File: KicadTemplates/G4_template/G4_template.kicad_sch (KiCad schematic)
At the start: 13 parts, among them J1 Conn_01x04_Female, SW1 SW_SPDT, U1 NUCLEO-G491RE

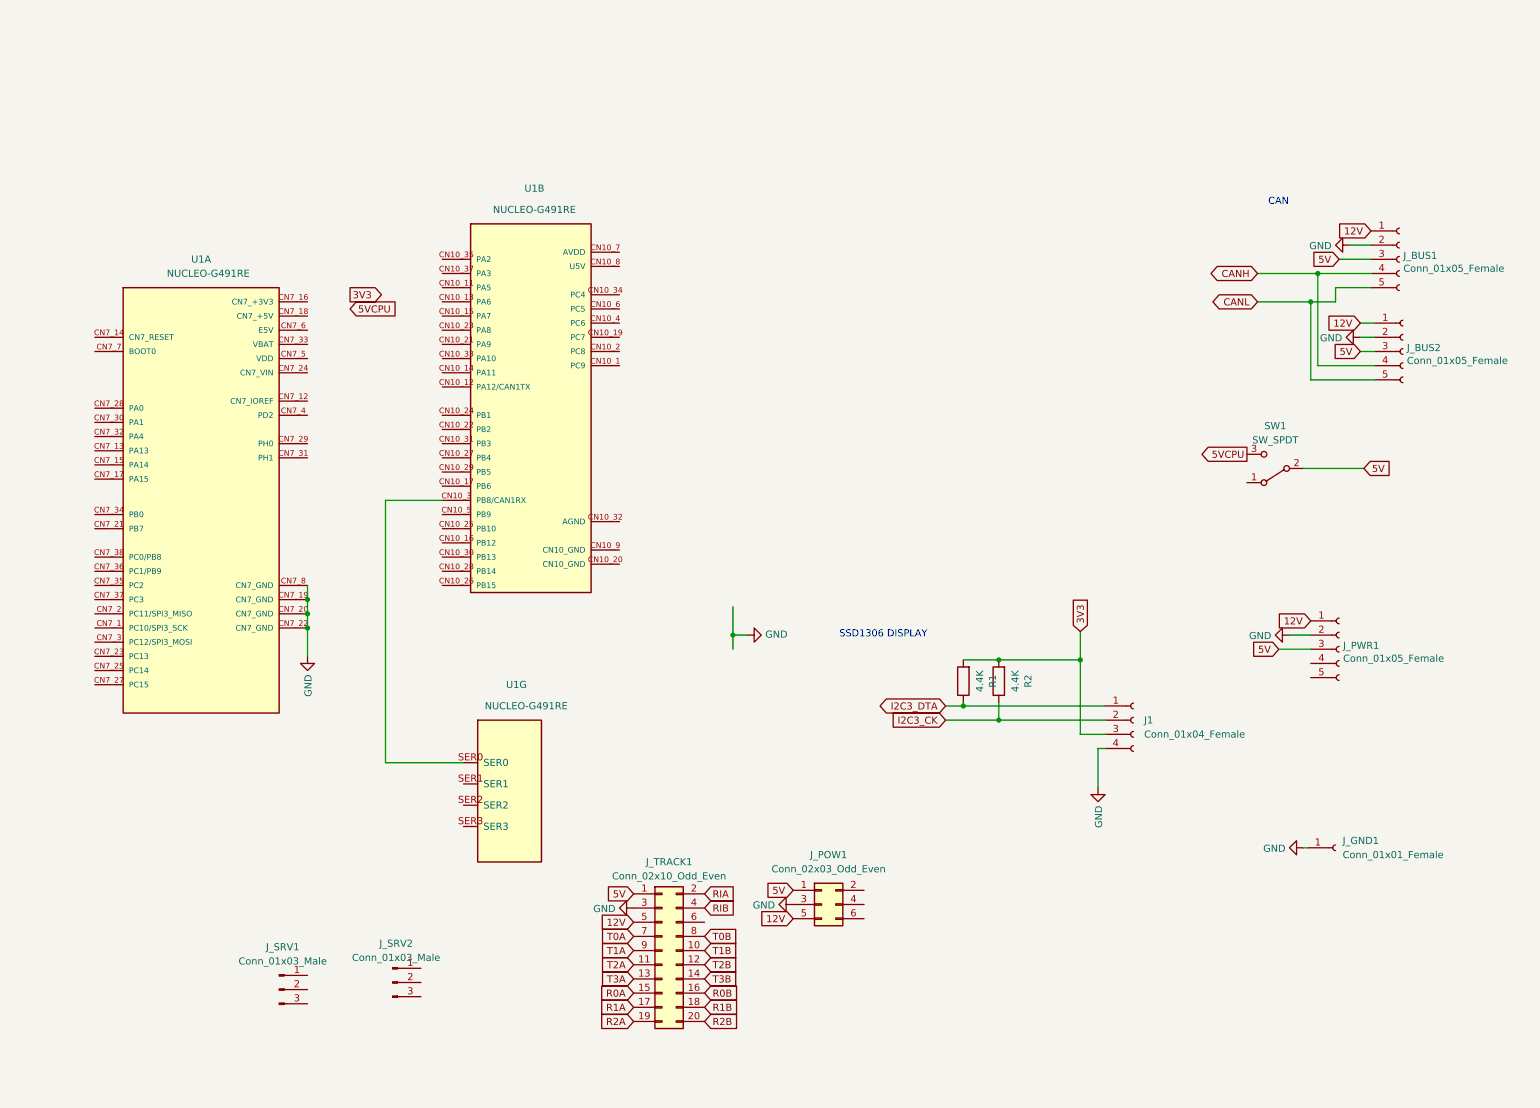
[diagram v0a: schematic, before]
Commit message: update spec
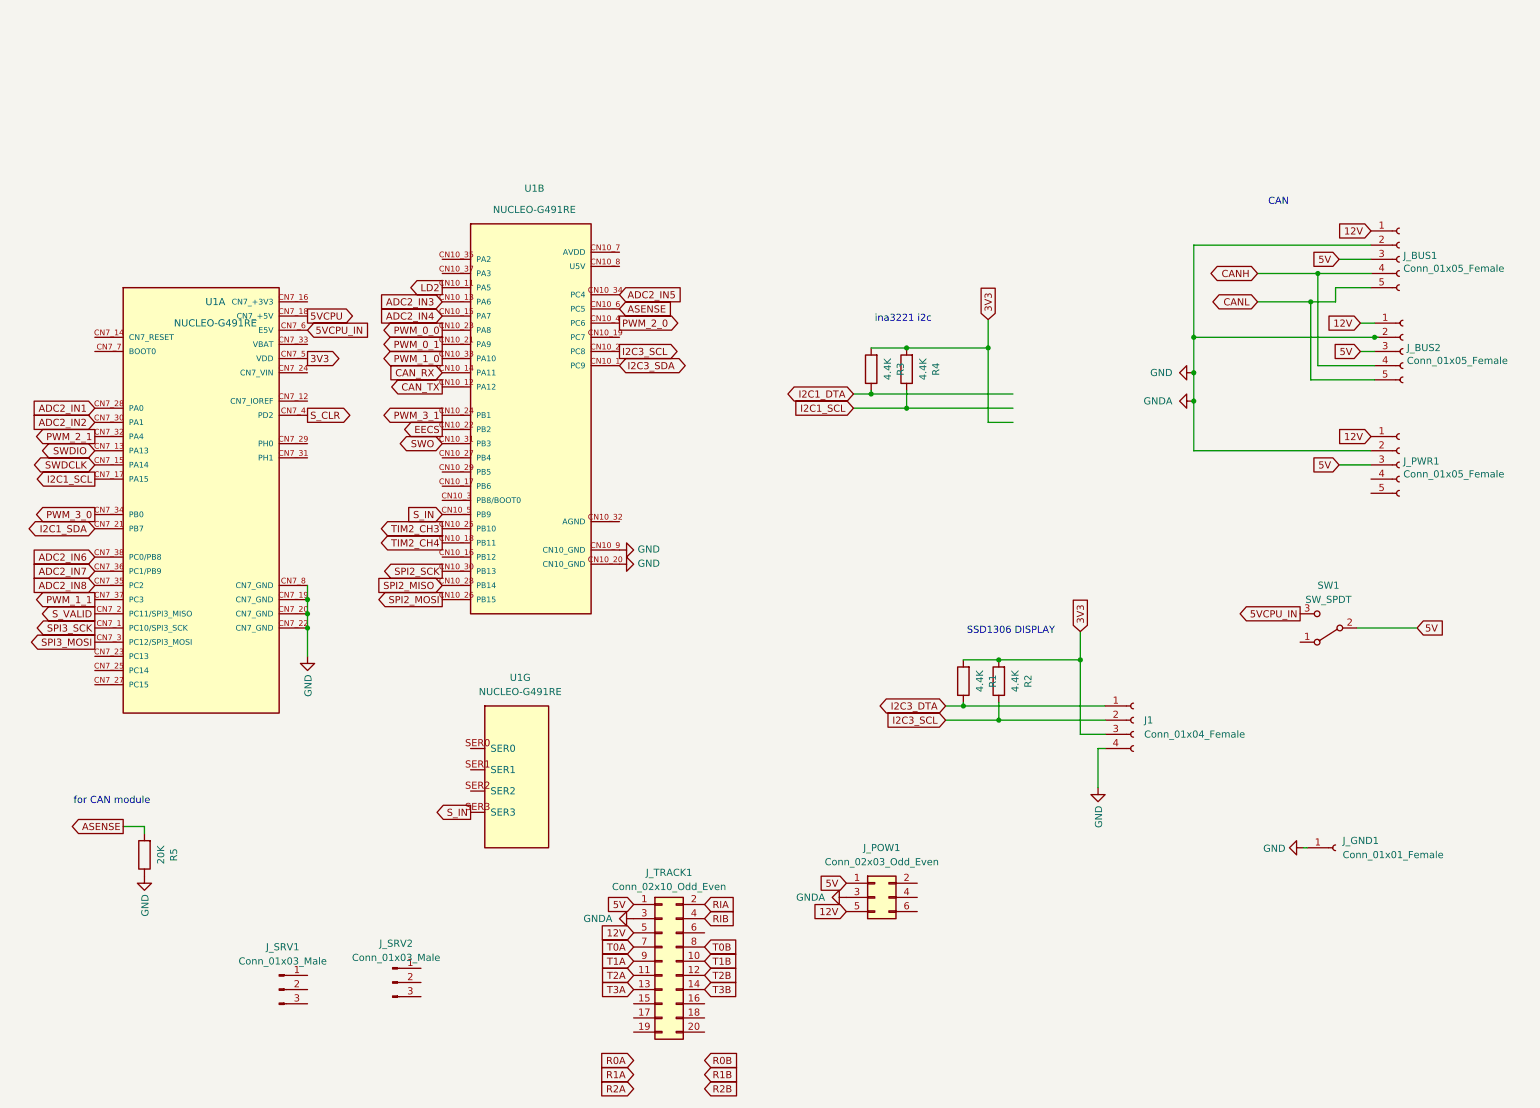
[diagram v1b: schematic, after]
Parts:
- added R3, R4: 4.4K, Resistor_THT:R_Axial_DIN0207_L6.3mm_D2.5mm_P7.62mm_Horizontal, symbol Device:R
- added R5: 20K, Resistor_THT:R_Axial_DIN0207_L6.3mm_D2.5mm_P7.62mm_Horizontal, symbol Device:R
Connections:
- net I2C3_CK is gone; now on net I2C3_SCL: J1.2 (Pin_2), R2.1
- net 3V3: now also U1.CN7_5 (VDD), R3.2, R4.2
- net 5VCPU: now also U1.CN7_18 (CN7_+5V); no longer SW1.3 (C)
- net GND: now also U1.CN10_20 (CN10_GND), U1.CN10_9 (CN10_GND), R5.1
- net R0A: no longer J_TRACK1.15 (Pin_15)
- net R0B: no longer J_TRACK1.16 (Pin_16)
- net R1A: no longer J_TRACK1.17 (Pin_17)
- net R1B: no longer J_TRACK1.18 (Pin_18)
- net R2A: no longer J_TRACK1.19 (Pin_19)
- net R2B: no longer J_TRACK1.20 (Pin_20)
- net at U1.SER0: no longer U1.CN10_3 (PB8/CAN1RX)
- net S_IN: now reaches U1.SER3
- net S_IN: now also U1.CN10_5 (PB9)
- net I2C3_SDA: now reaches U1.CN10_1 (PC9)
- net LD2: now reaches U1.CN10_11 (PA5)
- net CAN_TX: now reaches U1.CN10_12 (PA12)
- net ADC2_IN3: now reaches U1.CN10_13 (PA6)
- net CAN_RX: now reaches U1.CN10_14 (PA11)
- net ADC2_IN4: now reaches U1.CN10_15 (PA7)
- net I2C3_SCL: now reaches U1.CN10_2 (PC8)
- net PWM_0_1: now reaches U1.CN10_21 (PA9)
- net EECS: now reaches U1.CN10_22 (PB2)
- net PWM_0_0: now reaches U1.CN10_23 (PA8)
- net PWM_3_1: now reaches U1.CN10_24 (PB1)
- net TIM2_CH3: now reaches U1.CN10_25 (PB10)
- net SPI2_MOSI: now reaches U1.CN10_26 (PB15)
- net SPI2_MISO: now reaches U1.CN10_28 (PB14)
- net SPI2_SCK: now reaches U1.CN10_30 (PB13)
- net SWO: now reaches U1.CN10_31 (PB3)
- net PWM_1_0: now reaches U1.CN10_33 (PA10)
- net ADC2_IN5: now reaches U1.CN10_34 (PC4)
- net PWM_2_0: now reaches U1.CN10_4 (PC6)
- net ASENSE: now reaches U1.CN10_6 (PC5)
- net ASENSE: now also R5.2
- net SPI3_SCK: now reaches U1.CN7_1 (PC10/SPI3_SCK)
- net SWDIO: now reaches U1.CN7_13 (PA13)
- net SWDCLK: now reaches U1.CN7_15 (PA14)
- net I2C1_SCL: now reaches U1.CN7_17 (PA15)
- net I2C1_SCL: now also R4.1
- net S_VALID: now reaches U1.CN7_2 (PC11/SPI3_MISO)
- net I2C1_SDA: now reaches U1.CN7_21 (PB7)
- net ADC2_IN1: now reaches U1.CN7_28 (PA0)
- net SPI3_MOSI: now reaches U1.CN7_3 (PC12/SPI3_MOSI)
- net ADC2_IN2: now reaches U1.CN7_30 (PA1)
- net PWM_2_1: now reaches U1.CN7_32 (PA4)
- net PWM_3_0: now reaches U1.CN7_34 (PB0)
- net ADC2_IN8: now reaches U1.CN7_35 (PC2)
- net ADC2_IN7: now reaches U1.CN7_36 (PC1/PB9)
- net PWM_1_1: now reaches U1.CN7_37 (PC3)
- net ADC2_IN6: now reaches U1.CN7_38 (PC0/PB8)
- net S_CLR: now reaches U1.CN7_4 (PD2)
- net 5VCPU_IN: now reaches U1.CN7_6 (E5V)
- net 5VCPU_IN: now also SW1.3 (C)
- new net I2C1_DTA: R3.1
- new net TIM2_CH4: U1.CN10_18 (PB11)
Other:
- note added: "for CAN module"
- note added: "ina3221 i2c"
- company: (none) -> DBN
- title: (none) -> Template G4 V2
- moved on the sheet: J_POW1, J_PWR1, J_TRACK1, SW1, U1G
